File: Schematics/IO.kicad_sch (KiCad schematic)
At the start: 1 part

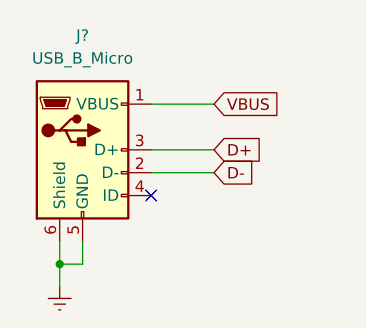
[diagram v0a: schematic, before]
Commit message: BOM + Motor Controllers
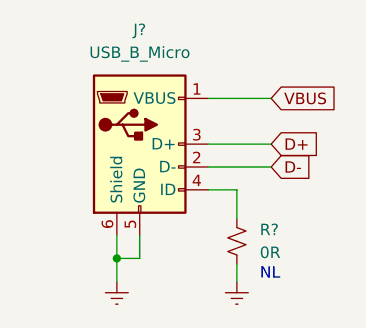
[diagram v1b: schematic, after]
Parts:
- added R?: 0R, symbol Device:R_Small_US
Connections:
- net Earth: now also R?.2
- net at J?.4 (ID): now also R?.1
- no-connect marks 1 -> 0
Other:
- note added: "NL"
- moved on the sheet: J?
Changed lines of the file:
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@@
 (kicad_sch (version 20211123) (generator eeschema)
   (paper "A4")
-  (junction (at 64.135 73.66) (diameter 0) (color 0 0 0 0)
+  (junction (at 70.485 73.025) (diameter 0) (color 0 0 0 0)
   )
-  (no_connect (at 74.295 66.04))
-  (wire (pts (xy 74.295 55.88) (xy 81.28 55.88))
+  (wire (pts (xy 80.645 55.245) (xy 87.63 55.245))
     (stroke (width 0) (type default) (color 0 0 0 0))
   )
-  (wire (pts (xy 74.295 60.96) (xy 81.28 60.96))
+  (wire (pts (xy 80.645 65.405) (xy 83.82 65.405))
     (stroke (width 0) (type default) (color 0 0 0 0))
   )
-  (wire (pts (xy 64.135 73.66) (xy 64.135 71.12))
+  (wire (pts (xy 80.645 60.325) (xy 87.63 60.325))
     (stroke (width 0) (type default) (color 0 0 0 0))
   )
-  (wire (pts (xy 64.135 76.2) (xy 64.135 73.66))
+  (wire (pts (xy 70.485 73.025) (xy 70.485 70.485))
     (stroke (width 0) (type default) (color 0 0 0 0))
   )
-  (wire (pts (xy 64.135 73.66) (xy 66.675 73.66))
+  (wire (pts (xy 70.485 75.565) (xy 70.485 73.025))
     (stroke (width 0) (type default) (color 0 0 0 0))
   )
-  (wire (pts (xy 74.295 63.5) (xy 81.28 63.5))
+  (wire (pts (xy 83.82 73.66) (xy 83.82 75.565))
     (stroke (width 0) (type default) (color 0 0 0 0))
   )
-  (wire (pts (xy 66.675 73.66) (xy 66.675 71.12))
+  (wire (pts (xy 83.82 65.405) (xy 83.82 68.58))
     (stroke (width 0) (type default) (color 0 0 0 0))
   )
-  (global_label "D+" (shape input) (at 81.28 60.96 0) (fields_autoplaced)
+  (wire (pts (xy 70.485 73.025) (xy 73.025 73.025))
+    (stroke (width 0) (type default) (color 0 0 0 0))
+  )
+  (wire (pts (xy 80.645 62.865) (xy 87.63 62.865))
+    (stroke (width 0) (type default) (color 0 0 0 0))
+  )
+  (wire (pts (xy 73.025 73.025) (xy 73.025 70.485))
+    (stroke (width 0) (type default) (color 0 0 0 0))
+  )
+  (text "NL" (at 86.36 75.565 0)
+    (effects (font (size 1.27 1.27)) (justify left bottom))
+  )
+  (global_label "D+" (shape input) (at 87.63 60.325 0) (fields_autoplaced)
     (effects (font (size 1.27 1.27)) (justify left))
-    (property "Intersheet References" "${INTERSHEET_REFS}" (id 0) (at 86.5355 60.8806 0)
+    (property "Intersheet References" "${INTERSHEET_REFS}" (id 0) (at 92.8855 60.2456 0)
       (effects (font (size 1.27 1.27)) (justify left) hide)
     )
   )
-  (global_label "VBUS" (shape input) (at 81.28 55.88 0) (fields_autoplaced)
+  (global_label "VBUS" (shape input) (at 87.63 55.245 0) (fields_autoplaced)
     (effects (font (size 1.27 1.27)) (justify left))
-    (property "Intersheet References" "${INTERSHEET_REFS}" (id 0) (at 88.5917 55.8006 0)
+    (property "Intersheet References" "${INTERSHEET_REFS}" (id 0) (at 94.9417 55.1656 0)
       (effects (font (size 1.27 1.27)) (justify left) hide)
     )
   )
-  (global_label "D-" (shape input) (at 81.28 63.5 0) (fields_autoplaced)
+  (global_label "D-" (shape input) (at 87.63 62.865 0) (fields_autoplaced)
     (effects (font (size 1.27 1.27)) (justify left))
-    (property "Intersheet References" "${INTERSHEET_REFS}" (id 0) (at 86.5355 63.4206 0)
+    (property "Intersheet References" "${INTERSHEET_REFS}" (id 0) (at 92.8855 62.7856 0)
       (effects (font (size 1.27 1.27)) (justify left) hide)
     )
   )
-  (symbol (lib_id "Connector:USB_B_Micro") (at 66.675 60.96 0) (unit 1)
+  (symbol (lib_id "Device:R_Small_US") (at 83.82 71.12 0) (unit 1)
     (in_bom yes) (on_board yes) (fields_autoplaced)
-    (property "Reference" "J?" (id 0) (at 66.675 48.26 0))
-    (property "Value" "USB_B_Micro" (id 1) (at 66.675 50.8 0))
-    (property "Footprint" "" (id 2) (at 70.485 62.23 0)
+    (property "Reference" "R?" (id 0) (at 86.36 69.8499 0)
+      (effects (font (size 1.27 1.27)) (justify left))
+    )
+    (property "Value" "0R" (id 1) (at 86.36 72.3899 0)
+      (effects (font (size 1.27 1.27)) (justify left))
+    )
+    (property "Footprint" "" (id 2) (at 83.82 71.12 0)
       (effects (font (size 1.27 1.27)) hide)
     )
-    (property "Datasheet" "~" (id 3) (at 70.485 62.23 0)
+    (property "Datasheet" "~" (id 3) (at 83.82 71.12 0)
+      (effects (font (size 1.27 1.27)) hide)
+    )
+    (pin "1")
+    (pin "2")
+  )
+  (symbol (lib_id "power:Earth") (at 83.82 75.565 0) (unit 1)
+    (in_bom yes) (on_board yes) (fields_autoplaced)
+    (property "Reference" "#PWR?" (id 0) (at 83.82 81.915 0)
+      (effects (font (size 1.27 1.27)) hide)
+    )
+    (property "Value" "Earth" (id 1) (at 83.82 79.375 0)
+      (effects (font (size 1.27 1.27)) hide)
+    )
+    (property "Footprint" "" (id 2) (at 83.82 75.565 0)
+      (effects (font (size 1.27 1.27)) hide)
+    )
+    (property "Datasheet" "~" (id 3) (at 83.82 75.565 0)
+      (effects (font (size 1.27 1.27)) hide)
+    )
+    (pin "1")
+  )
+  (symbol (lib_id "Connector:USB_B_Micro") (at 73.025 60.325 0) (unit 1)
+    (in_bom yes) (on_board yes) (fields_autoplaced)
+    (property "Reference" "J?" (id 0) (at 73.025 47.625 0))
+    (property "Value" "USB_B_Micro" (id 1) (at 73.025 50.165 0))
+    (property "Footprint" "" (id 2) (at 76.835 61.595 0)
+      (effects (font (size 1.27 1.27)) hide)
+    )
+    (property "Datasheet" "~" (id 3) (at 76.835 61.595 0)
       (effects (font (size 1.27 1.27)) hide)
     )
@@
     (pin "6")
   )
-  (symbol (lib_id "power:Earth") (at 64.135 76.2 0) (unit 1)
+  (symbol (lib_id "power:Earth") (at 70.485 75.565 0) (unit 1)
     (in_bom yes) (on_board yes) (fields_autoplaced)
-    (property "Reference" "#PWR?" (id 0) (at 64.135 82.55 0)
+    (property "Reference" "#PWR?" (id 0) (at 70.485 81.915 0)
       (effects (font (size 1.27 1.27)) hide)
     )
-    (property "Value" "Earth" (id 1) (at 64.135 80.01 0)
+    (property "Value" "Earth" (id 1) (at 70.485 79.375 0)
       (effects (font (size 1.27 1.27)) hide)
     )
-    (property "Footprint" "" (id 2) (at 64.135 76.2 0)
+    (property "Footprint" "" (id 2) (at 70.485 75.565 0)
       (effects (font (size 1.27 1.27)) hide)
     )
-    (property "Datasheet" "~" (id 3) (at 64.135 76.2 0)
+    (property "Datasheet" "~" (id 3) (at 70.485 75.565 0)
       (effects (font (size 1.27 1.27)) hide)
     )
